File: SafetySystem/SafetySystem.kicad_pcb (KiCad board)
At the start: 2 copper layers, 70 x 60 mm, 96 parts, among them J1 Screw_Terminal_01x02, J10 Screw_Terminal_01x02, J2 Screw_Terminal_01x02, J3 Screw_Terminal_01x02, J4 AVR-ISP-10, J5 Screw_Terminal_01x02, J6 Screw_Terminal_01x02, J7 Screw_Terminal_01x02, J8 Screw_Terminal_01x02, J9 Screw_Terminal_01x02, Q1 Q_PMOS_GSD, Q10 Q_NMOS_GSD, Q11 Q_NMOS_GSD, Q12 Q_NMOS_GSD, Q2 Q_PMOS_GSD, Q3 Q_PMOS_GSD, Q4 Q_NMOS_GSD, Q5 Q_NMOS_GSD, Q6 Q_NMOS_GSD, Q7 Q_NMOS_GSD, Q8 Q_NMOS_GSD, Q9 Q_NMOS_GSD, SW2 SW_Push, SW3 SW_Push, SW4 SW_Push, U1 ST1S10PHR, U2 MQ-8, U3 ATmega8A-AU, U4 LTV-817S, U5 LTV-817S, Y1 8Mhz

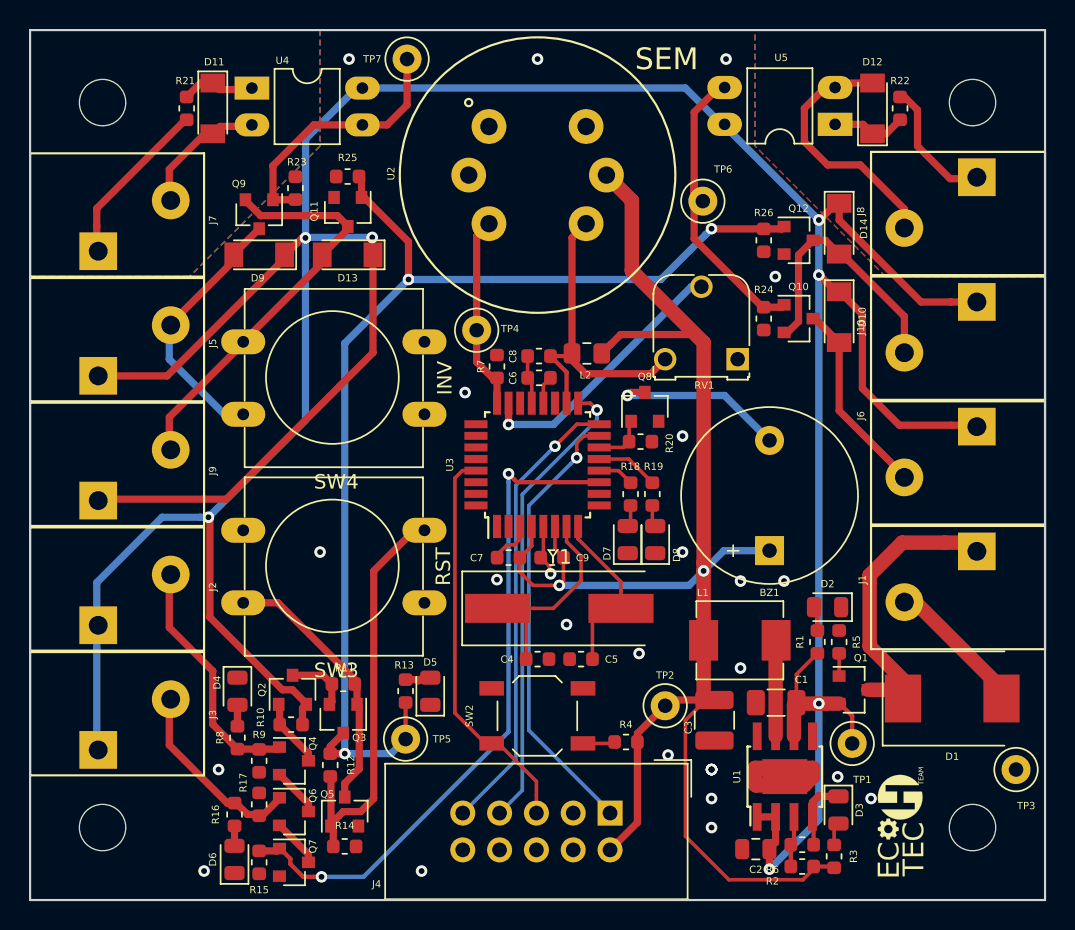
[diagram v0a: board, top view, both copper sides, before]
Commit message: Adding gerbers
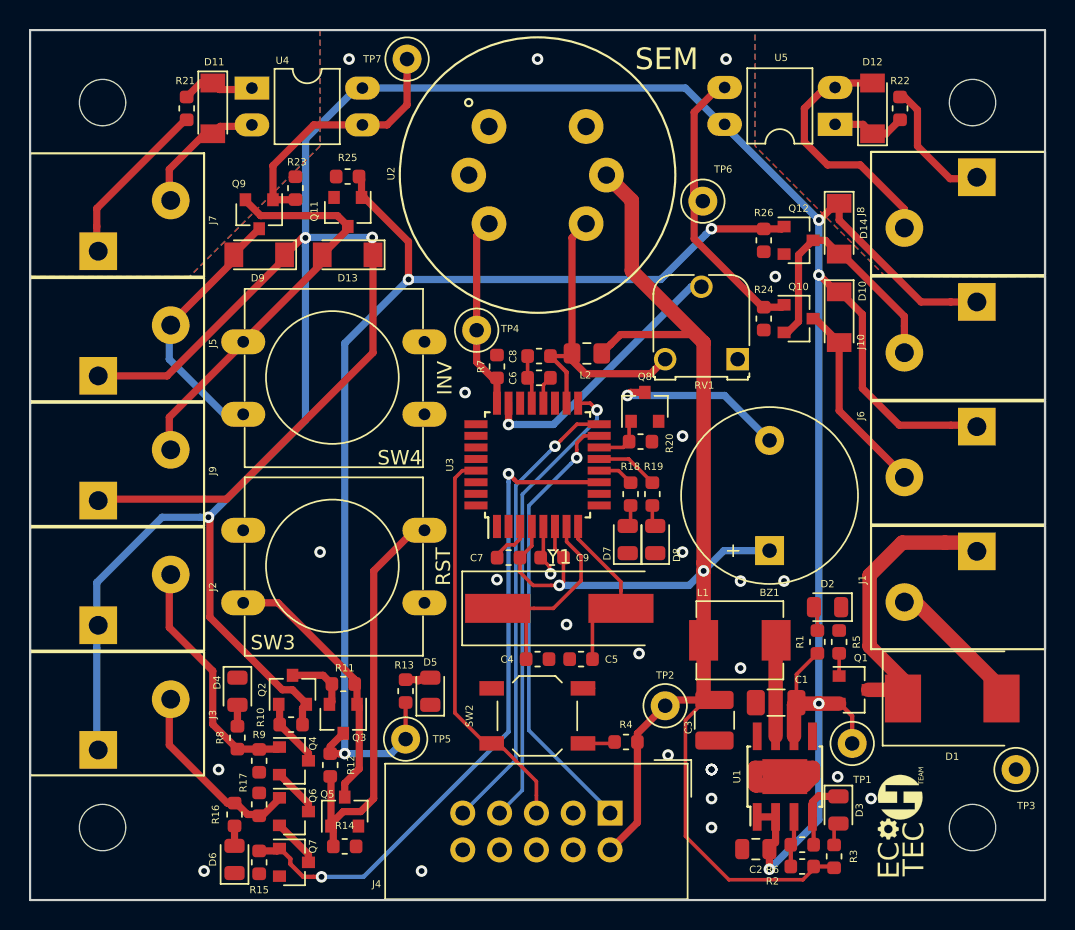
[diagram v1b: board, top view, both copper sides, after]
